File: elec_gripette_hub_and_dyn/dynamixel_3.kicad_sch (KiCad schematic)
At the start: 26 parts, among them J4 Dynamixel-3, J5 Dynamixel-3, J9 Dynamixel-3, Q1 MMBT3906, U3 CH343P, U4 SN74LVC1G125DBV, U5 SN74LVC1G126DBVR

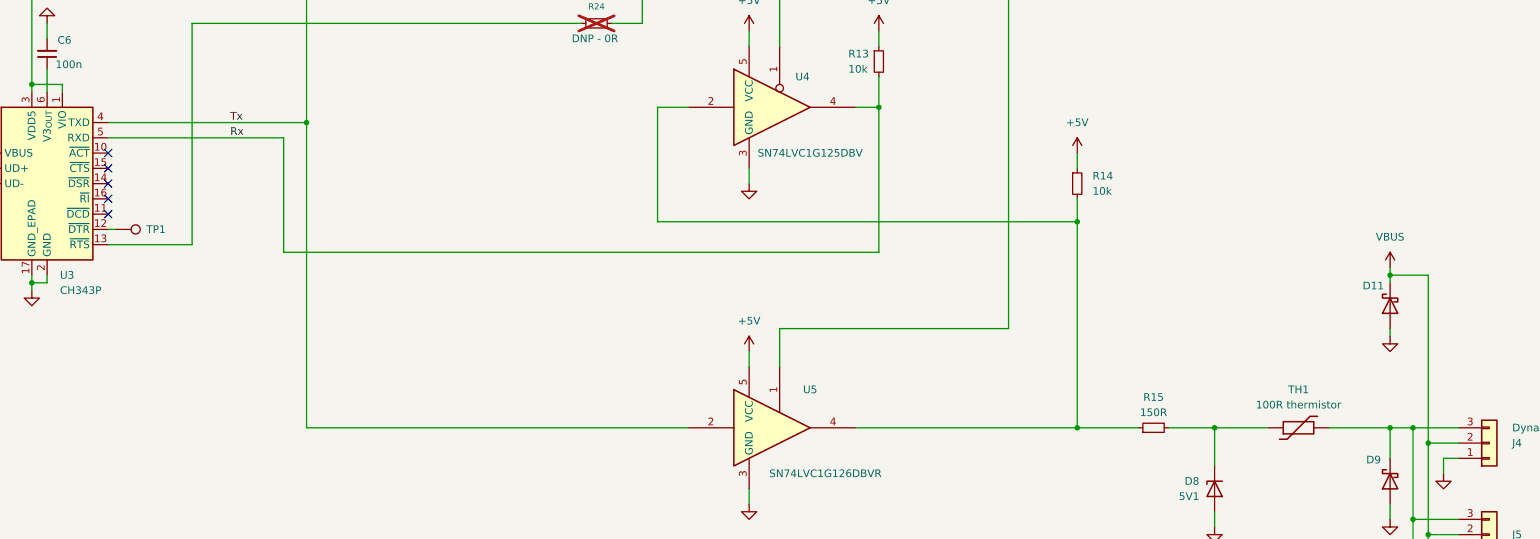
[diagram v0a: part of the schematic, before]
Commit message: [update] SCH B1-RC1
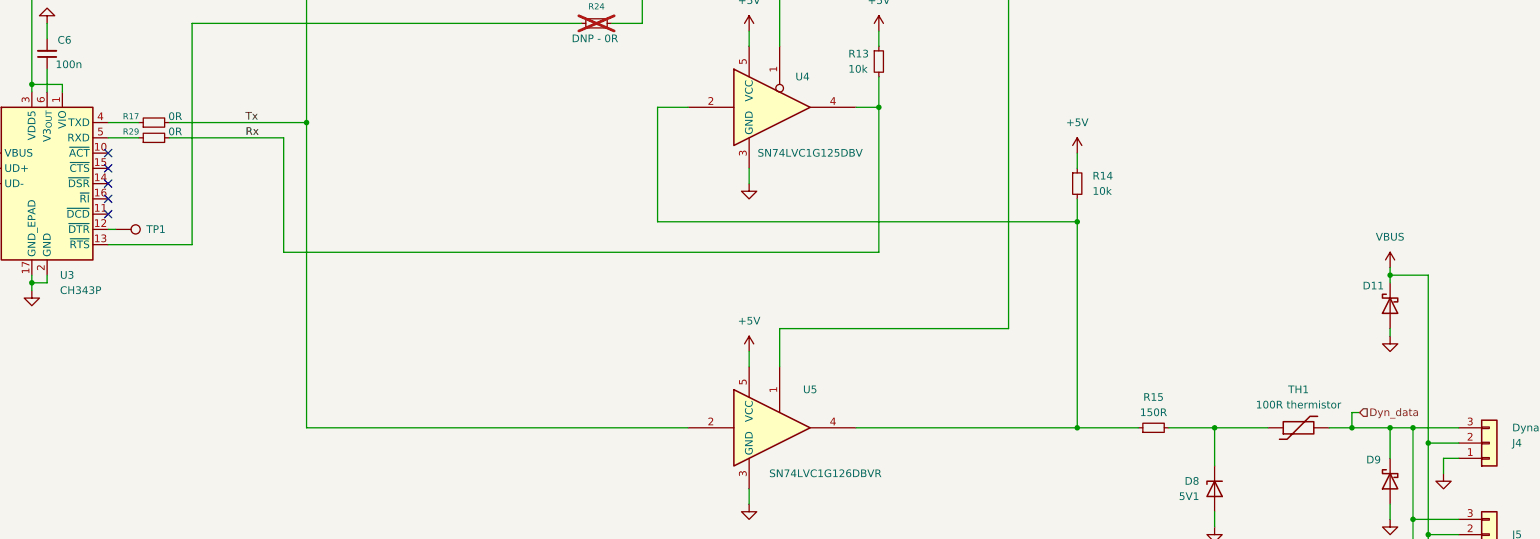
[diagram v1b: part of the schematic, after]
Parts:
- added R17, R29: 0R, Resistor_SMD:R_0402_1005Metric, symbol Device:R_Small
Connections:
- net Rx: now also R29.2; no longer U3.5 (RXD)
- net Tx: now also R17.2; no longer U3.4 (TXD)
- net Dyn_data: now reaches D9.1 (K), J4.3 (Pin_3), J5.3 (Pin_3), J9.3 (Pin_3), TH1.2
- new net: R29.1, U3.5 (RXD)
- new net: R17.1, U3.4 (TXD)
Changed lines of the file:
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@@
 	(title_block
 		(title "Grippette - USB hub and Dynamixel device")
-		(date "2026-04-16")
-		(rev "A1")
+		(date "2026-05-27")
+		(rev "B1")
 		(company "Pollen Robotics/HF")
 	)
@@
 	)
 	(junction
+		(at 311.15 173.99)
+		(diameter 0)
+		(color 0 0 0 0)
+	)
+	(junction
 		(at 215.9 88.9)
 		(diameter 0)
@@
 	(wire
 		(pts
+			(xy 114.3 123.19) (xy 137.16 123.19)
+		)
+		(stroke
+			(width 0)
+			(type default)
+		)
+	)
+	(wire
+		(pts
 			(xy 328.93 189.23) (xy 321.31 189.23)
 		)
@@
 	(wire
 		(pts
+			(xy 114.3 125.73) (xy 133.35 125.73)
+		)
+		(stroke
+			(width 0)
+			(type default)
+		)
+	)
+	(wire
+		(pts
 			(xy 207.01 205.74) (xy 207.01 208.28)
 		)
@@
 	(wire
 		(pts
-			(xy 104.14 125.73) (xy 133.35 125.73)
+			(xy 104.14 125.73) (xy 109.22 125.73)
 		)
 		(stroke
@@
 	(wire
 		(pts
-			(xy 307.34 173.99) (xy 317.5 173.99)
+			(xy 307.34 173.99) (xy 311.15 173.99)
 		)
 		(stroke
@@
 	(wire
 		(pts
+			(xy 312.42 171.45) (xy 311.15 171.45)
+		)
+		(stroke
+			(width 0)
+			(type default)
+		)
+	)
+	(wire
+		(pts
 			(xy 228.6 120.65) (xy 232.41 120.65)
 		)
@@
 	(wire
 		(pts
-			(xy 104.14 123.19) (xy 137.16 123.19)
+			(xy 104.14 123.19) (xy 109.22 123.19)
 		)
 		(stroke
@@
 	(wire
 		(pts
+			(xy 311.15 171.45) (xy 311.15 173.99)
+		)
+		(stroke
+			(width 0)
+			(type default)
+		)
+	)
+	(wire
+		(pts
 			(xy 91.44 101.6) (xy 91.44 116.84)
 		)
@@
 	(wire
 		(pts
+			(xy 311.15 173.99) (xy 317.5 173.99)
+		)
+		(stroke
+			(width 0)
+			(type default)
+		)
+	)
+	(wire
+		(pts
 			(xy 215.9 88.9) (xy 215.9 110.49)
 		)
@@
 	)
 	(label "Rx"
-		(at 124.46 125.73 0)
+		(at 127 125.73 0)
 		(effects
 			(font
@@
 	)
 	(label "Tx"
-		(at 124.46 123.19 0)
+		(at 127 123.19 0)
 		(effects
 			(font
@@
 		)
 	)
+	(hierarchical_label "Dyn_data"
+		(shape input)
+		(at 312.42 171.45 0)
+		(effects
+			(font
+				(size 1.27 1.27)
+			)
+			(justify left)
+		)
+	)
 	(symbol
 		(lib_id "Device:R_Small")
@@
 	)
 	(symbol
+		(lib_id "Device:R_Small")
+		(at 111.76 125.73 90)
+		(unit 1)
+		(exclude_from_sim no)
+		(in_bom yes)
+		(on_board yes)
+		(dnp no)
+		(property "Reference" "R29"
+			(at 107.95 124.714 90)
+			(effects
+				(font
+					(size 1.016 1.016)
+				)
+			)
+		)
+		(property "Value" "0R"
+			(at 115.316 124.714 90)
+			(effects
+				(font
+					(size 1.27 1.27)
+				)
+			)
+		)
+		(property "Footprint" "Resistor_SMD:R_0402_1005Metric"
+			(at 111.76 125.73 0)
+			(effects
+				(font
+					(size 1.27 1.27)
+				)
+				(hide yes)
+			)
+		)
+		(property "Datasheet" "~"
+			(at 111.76 125.73 0)
+			(effects
+				(font
+					(size 1.27 1.27)
+				)
+				(hide yes)
+			)
+		)
+		(property "Description" "Resistor, small symbol"
+			(at 111.76 125.73 0)
+			(effects
+				(font
+					(size 1.27 1.27)
+				)
+				(hide yes)
+			)
+		)
+		(property "LCSC Part" "C17168"
+			(at 111.76 125.73 90)
+			(effects
+				(font
+					(size 1.27 1.27)
+				)
+				(hide yes)
+			)
+		)
+		(pin "2"
+		)
+		(pin "1"
+		)
+		(instances
+			(project "elec_gripette_hub_and_dyn"
+				(path "/bc05f5da-608c-4912-90e4-36b13d989976/edad0453-e3dd-48f4-9e65-34ff832c5255"
+					(reference "R29")
+					(unit 1)
+				)
+			)
+		)
+	)
+	(symbol
 		(lib_id "power:GND")
 		(at 80.01 111.76 0)
@@
 					(unit 1)
 				)
+			)
+		)
+	)
+	(symbol
+		(lib_id "Device:R_Small")
+		(at 111.76 123.19 90)
+		(unit 1)
+		(exclude_from_sim no)
+		(in_bom yes)
+		(on_board yes)
+		(dnp no)
+		(property "Reference" "R17"
+			(at 107.95 122.174 90)
+			(effects
+				(font
+					(size 1.016 1.016)
+				)
+			)
+		)
+		(property "Value" "0R"
+			(at 115.316 122.174 90)
+			(effects
+				(font
+					(size 1.27 1.27)
+				)
+			)
+		)
+		(property "Footprint" "Resistor_SMD:R_0402_1005Metric"
+			(at 111.76 123.19 0)
+			(effects
+				(font
+					(size 1.27 1.27)
+				)
+				(hide yes)
+			)
+		)
+		(property "Datasheet" "~"
+			(at 111.76 123.19 0)
+			(effects
+				(font
+					(size 1.27 1.27)
+				)
+				(hide yes)
+			)
+		)
+		(property "Description" "Resistor, small symbol"
+			(at 111.76 123.19 0)
+			(effects
+				(font
+					(size 1.27 1.27)
+				)
+				(hide yes)
+			)
+		)
+		(property "LCSC Part" "C17168"
+			(at 111.76 123.19 90)
+			(effects
+				(font
+					(size 1.27 1.27)
+				)
+				(hide yes)
+			)
+		)
+		(pin "2"
+		)
+		(pin "1"
+		)
+		(instances
+			(project "elec_gripette_hub_and_dyn"
+				(path "/bc05f5da-608c-4912-90e4-36b13d989976/edad0453-e3dd-48f4-9e65-34ff832c5255"
+					(reference "R17")
+					(unit 1)
+				)
